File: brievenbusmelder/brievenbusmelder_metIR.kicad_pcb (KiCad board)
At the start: 2 copper layers, 29.5 x 16.8 mm, 9 parts, among them IC1 VCNL3030X01-GS08, J2 Conn_01x05_Male

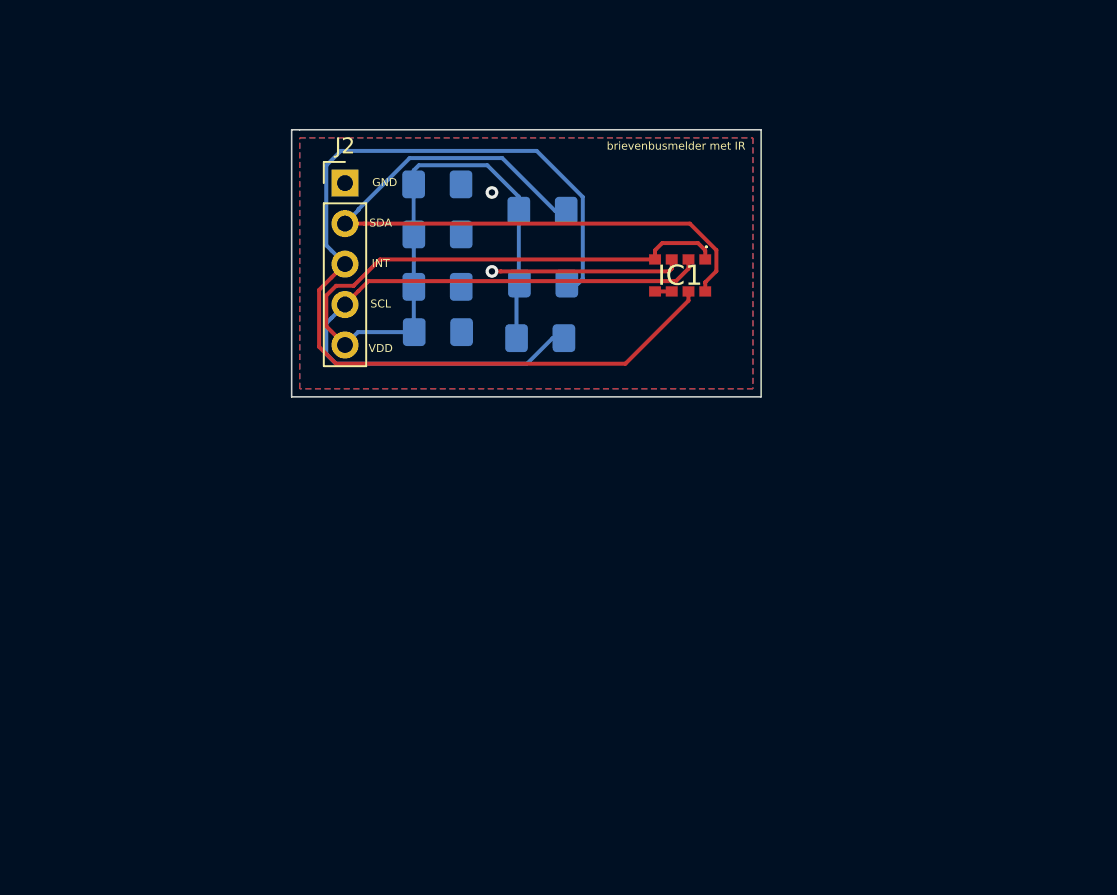
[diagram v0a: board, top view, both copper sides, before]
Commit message: Update brievenbusmelder_metIR.kicad_pcb
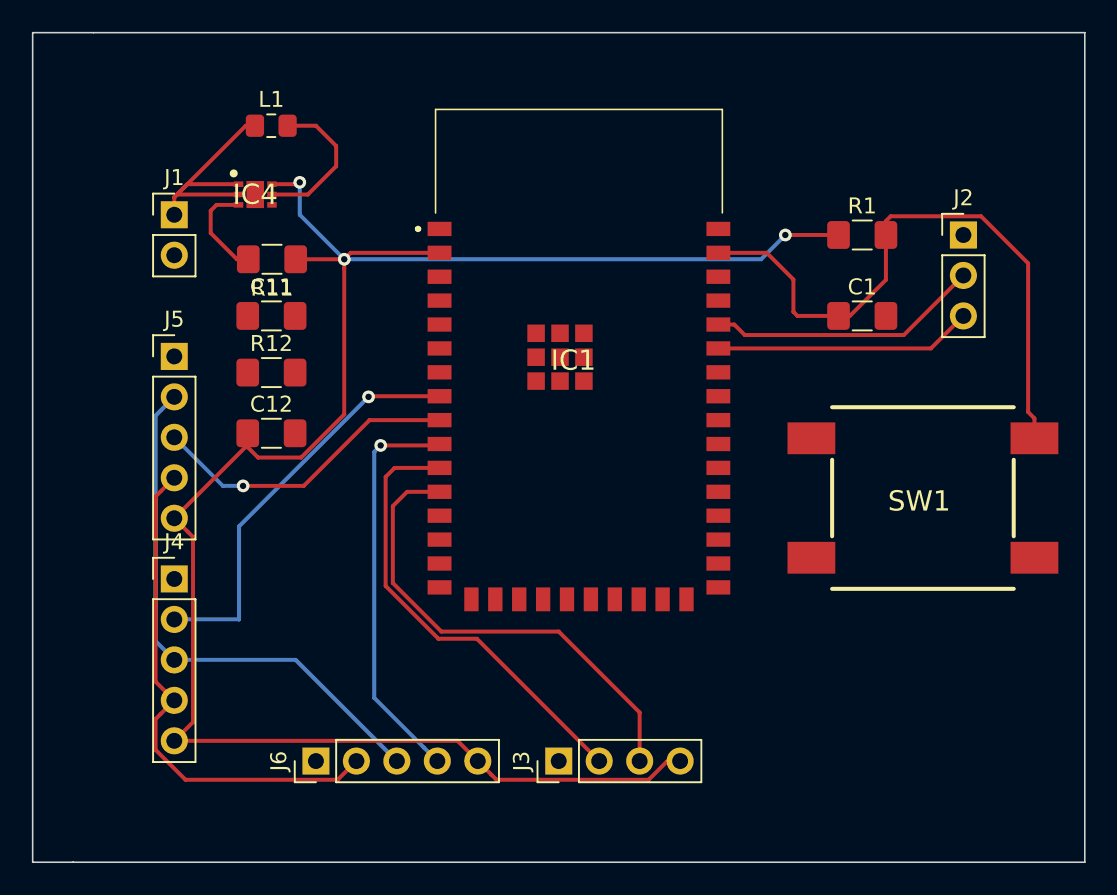
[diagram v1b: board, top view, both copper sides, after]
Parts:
- removed C2: 22µF, Capacitor_SMD:C_1206_3216Metric_Pad1.42x1.75mm_HandSolder
- removed C3, C5: 100nF, Capacitor_SMD:C_1206_3216Metric_Pad1.42x1.75mm_HandSolder
- removed C6: 10µF, Capacitor_SMD:C_1206_3216Metric_Pad1.42x1.75mm_HandSolder
- removed R4: 2.2k, Resistor_SMD:R_1206_3216Metric_Pad1.42x1.75mm_HandSolder
- removed R5: 2.2K, Resistor_SMD:R_1206_3216Metric_Pad1.42x1.75mm_HandSolder
- removed R6: 8.2K, Resistor_SMD:R_1206_3216Metric_Pad1.42x1.75mm_HandSolder
- added C1: 1µF, Capacitor_SMD:C_1206_3216Metric_Pad1.42x1.75mm_HandSolder, F.Cu at (118.1, 66.0)
- added C11: 10µF, Capacitor_SMD:C_1206_3216Metric_Pad1.42x1.75mm_HandSolder, F.Cu at (81.0, 66.0)
- added C12: 10µF, Capacitor_SMD:C_1206_3216Metric_Pad1.42x1.75mm_HandSolder, F.Cu at (81.0, 73.4)
- added IC4: ADP1607ACPZN001-R7, schakelende_voeding_1_7A:SON65P200X200X65-7N-D, F.Cu at (80.0, 58.4)
- added J1: Conn_01x02_Male, Connector_PinHeader_2.54mm:PinHeader_1x02_P2.54mm_Vertical, F.Cu at (74.9, 59.7)
- added J3: temp_con, Connector_PinHeader_2.54mm:PinHeader_1x04_P2.54mm_Vertical, F.Cu at (99.1, 94.0)
- added J4: opt_conn, Connector_PinHeader_2.54mm:PinHeader_1x05_P2.54mm_Vertical, F.Cu at (74.9, 82.5)
- added J5: IR_met_conn, Connector_PinHeader_2.54mm:PinHeader_1x05_P2.54mm_Vertical, F.Cu at (74.9, 68.6)
- added J6: IR_zonder_conn, Connector_PinHeader_2.54mm:PinHeader_1x05_P2.54mm_Vertical, F.Cu at (83.8, 94.0)
- added L1: 2.2µH, Inductor_SMD:L_0805_2012Metric_Pad1.15x1.40mm_HandSolder, F.Cu at (81.0, 54.1)
- added R1: 10k, Resistor_SMD:R_1206_3216Metric_Pad1.42x1.75mm_HandSolder, F.Cu at (118.1, 61.0)
- added R11: 27000, Resistor_SMD:R_1206_3216Metric_Pad1.42x1.75mm_HandSolder, F.Cu at (81.1, 62.5)
- added R12: 18000, Resistor_SMD:R_1206_3216Metric_Pad1.42x1.75mm_HandSolder, F.Cu at (81.0, 69.6)
- added SW1: SW_Push, Drukknop_OFF_(ON):Drukknop_OFF_(ON), F.Cu at (121.9, 77.5)
- IC1: value VCNL3030X01-GS08 -> ESP32-S2-WROOM_M22S2H3200PH3Q0_; footprint naderingssensor_metIR:VCNL3030X01GS08 -> ESP32S2WROOMM22S2H3200PH3Q0
- J2: value Conn_01x05_Male -> Conn_01x03_Male; footprint Connector_PinHeader_2.54mm:PinHeader_1x05_P2.54mm_Vertical -> Connector_PinHeader_2.54mm:PinHeader_1x03_P2.54mm_Vertical
- moved J2 39.0 mm to (124.5, 61.0)
- moved IC1 8.13 mm to (100.3, 68.6)
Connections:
- IC1 pad 1: Net-(C2-Pad1) -> GND
- IC1 pad 2: Net-(IC1-Pad2) -> Net-(C12-Pad1)
- IC1 pad 3: GND -> Net-(IC1-Pad3)
- IC1 pad 4: Net-(C2-Pad1) -> Net-(IC1-Pad4)
- IC1 pad 6: Net-(IC1-Pad5) -> Net-(IC1-Pad6)
- J2 pad 2: Net-(IC1-Pad8) -> Net-(IC1-Pad38)
- J2 pad 3: Net-(IC1-Pad7) -> Net-(IC1-Pad37)
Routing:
- net Net-(C12-Pad1): track 0.00 -> 122.1 mm, vias 0 -> 3
- net Net-(IC1-Pad7): track 62.3 -> 0.00 mm
- net Net-(C2-Pad1): track 61.2 -> 0.00 mm
- net Net-(IC1-Pad2): track 42.5 -> 0.00 mm
- net Net-(C1-Pad1): track 0.00 -> 39.4 mm
- net Net-(J4-Pad3): track 0.00 -> 34.1 mm
- net Net-(J4-Pad4): track 0.00 -> 32.4 mm
- net Net-(IC1-Pad12): track 0.00 -> 30.0 mm
- net Net-(IC1-Pad11): track 0.00 -> 28.4 mm
- net Net-(IC1-Pad10): track 0.00 -> 25.3 mm, vias 0 -> 1
- net Net-(IC1-Pad9): track 0.00 -> 19.6 mm, vias 0 -> 1
- net Net-(IC1-Pad8): track 43.9 -> 25.9 mm, vias 0 -> 1
- net Net-(IC1-Pad38): track 0.00 -> 17.2 mm
- net Net-(C11-Pad1): track 0.00 -> 16.5 mm
- net Net-(IC1-Pad37): track 0.00 -> 16.2 mm
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- removed copper zone on B.Cu, net GND
- removed copper zone on F.Cu, net GND
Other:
- board size 29.5 x 16.8 mm -> 66 x 52.1 mm
- board text removed: "GND"
- board text removed: "INT"
- board text removed: "SCL"
- board text removed: "SDA"
- board text removed: "VDD"
- board text removed: "brievenbusmelder met IR"
